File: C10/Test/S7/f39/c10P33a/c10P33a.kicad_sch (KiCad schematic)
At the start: 5 parts

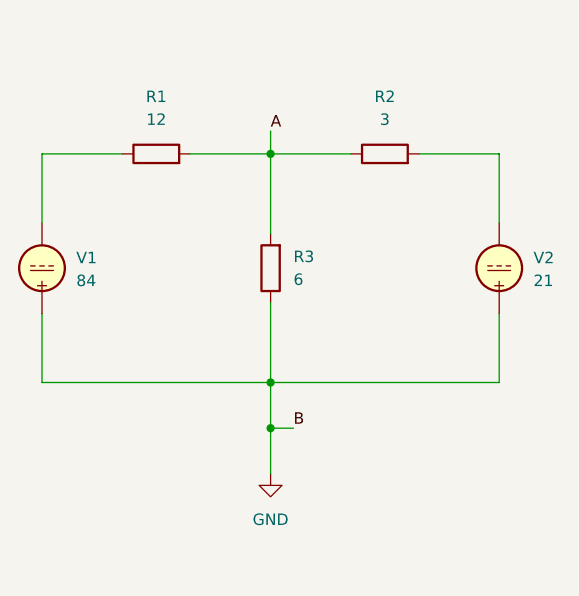
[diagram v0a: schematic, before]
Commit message: additiona upload Chapter 10
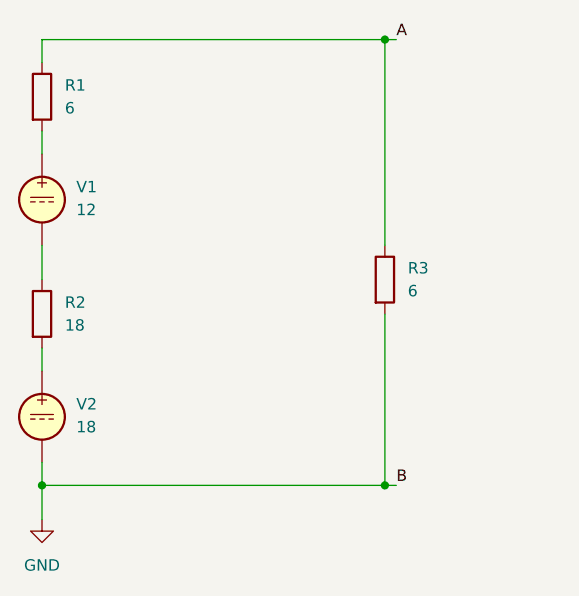
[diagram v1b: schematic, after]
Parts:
- R1: value 12 -> 6
- R2: value 3 -> 18
- V1: value 84 -> 12
- V2: value 21 -> 18
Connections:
- net A: now also R1.1, R3.1; no longer R1.2, R2.1, R3.2
- net GND: now also R3.2, V2.2; no longer R3.1, V1.1, V2.1
- net at V1.2: now also R2.1; no longer R1.1
- net at R2.2: now also V2.1; no longer V2.2
- new net: R1.2, V1.1
